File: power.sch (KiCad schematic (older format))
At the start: 21 parts

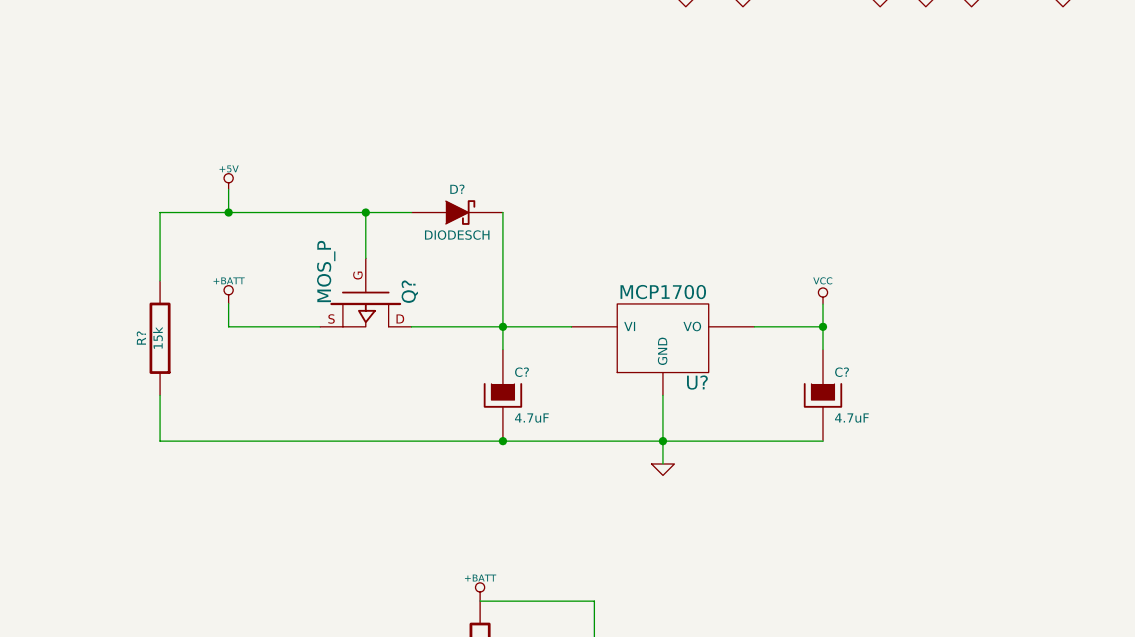
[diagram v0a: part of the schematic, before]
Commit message: Add power switch
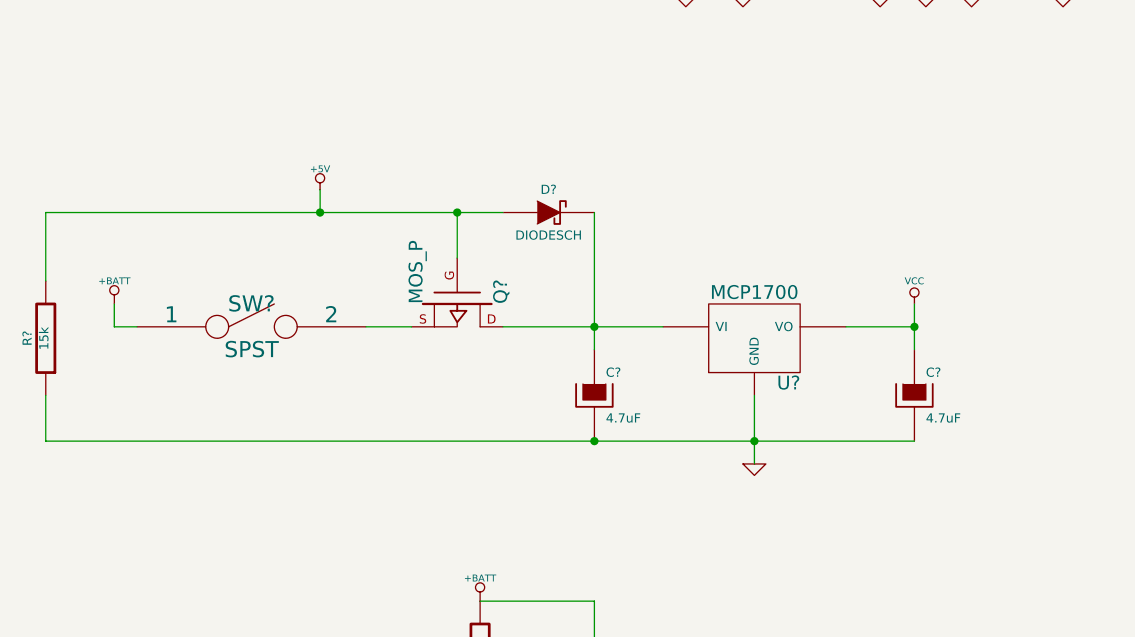
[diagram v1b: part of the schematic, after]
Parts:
- added SW?: SPST, symbol SPST
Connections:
- net +BATT: now also SW?.1; no longer Q?.S
- new net: Q?.S, SW?.2
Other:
- moved on the sheet: C?, D?, Q?, R?, U?
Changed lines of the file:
@@
 L MOS_P Q?
 U 1 1 54E64290
-P 2200 3900
-F 0 "Q?" H 2200 4090 60  0000 R CNN
-F 1 "MOS_P" H 2200 3720 60  0000 R CNN
-F 2 "" H 2200 3900 60  0000 C CNN
-F 3 "" H 2200 3900 60  0000 C CNN
-	1    2200 3900
+P 2600 3900
+F 0 "Q?" H 2600 4090 60  0000 R CNN
+F 1 "MOS_P" H 2600 3720 60  0000 R CNN
+F 2 "" H 2600 3900 60  0000 C CNN
+F 3 "" H 2600 3900 60  0000 C CNN
+	1    2600 3900
 	0    1    1    0
 $EndComp
@@
 L +BATT #PWR?
 U 1 1 54E64297
-P 1600 3900
-F 0 "#PWR?" H 1600 3850 20  0001 C CNN
-F 1 "+BATT" H 1600 4000 30  0000 C CNN
-F 2 "" H 1600 3900 60  0000 C CNN
-F 3 "" H 1600 3900 60  0000 C CNN
-	1    1600 3900
+P 1100 3900
+F 0 "#PWR?" H 1100 3850 20  0001 C CNN
+F 1 "+BATT" H 1100 4000 30  0000 C CNN
+F 2 "" H 1100 3900 60  0000 C CNN
+F 3 "" H 1100 3900 60  0000 C CNN
+	1    1100 3900
 	1    0    0    -1
 $EndComp
@@
 L CP C?
 U 1 1 54E6429D
-P 2800 4300
-F 0 "C?" H 2850 4400 40  0000 L CNN
-F 1 "4.7uF" H 2850 4200 40  0000 L CNN
-F 2 "" H 2900 4150 30  0000 C CNN
-F 3 "" H 2800 4300 300 0000 C CNN
-	1    2800 4300
+P 3200 4300
+F 0 "C?" H 3250 4400 40  0000 L CNN
+F 1 "4.7uF" H 3250 4200 40  0000 L CNN
+F 2 "" H 3300 4150 30  0000 C CNN
+F 3 "" H 3200 4300 300 0000 C CNN
+	1    3200 4300
 	1    0    0    -1
 $EndComp
@@
 L DIODESCH D?
 U 1 1 54E642A4
-P 2600 3500
-F 0 "D?" H 2600 3600 40  0000 C CNN
-F 1 "DIODESCH" H 2600 3400 40  0000 C CNN
-F 2 "" H 2600 3500 60  0000 C CNN
-F 3 "" H 2600 3500 60  0000 C CNN
-	1    2600 3500
+P 3000 3500
+F 0 "D?" H 3000 3600 40  0000 C CNN
+F 1 "DIODESCH" H 3000 3400 40  0000 C CNN
+F 2 "" H 3000 3500 60  0000 C CNN
+F 3 "" H 3000 3500 60  0000 C CNN
+	1    3000 3500
 	1    0    0    -1
 $EndComp
@@
 L MCP1700 U?
 U 1 1 54E642AB
-P 3500 4050
-F 0 "U?" H 3650 3854 60  0000 C CNN
-F 1 "MCP1700" H 3500 4250 60  0000 C CNN
-F 2 "" H 3500 4050 60  0000 C CNN
-F 3 "" H 3500 4050 60  0000 C CNN
-	1    3500 4050
+P 3900 4050
+F 0 "U?" H 4050 3854 60  0000 C CNN
+F 1 "MCP1700" H 3900 4250 60  0000 C CNN
+F 2 "" H 3900 4050 60  0000 C CNN
+F 3 "" H 3900 4050 60  0000 C CNN
+	1    3900 4050
 	1    0    0    -1
 $EndComp
@@
 L VCC #PWR?
 U 1 1 54E642B2
-P 4200 3900
-F 0 "#PWR?" H 4200 4000 30  0001 C CNN
-F 1 "VCC" H 4200 4000 30  0000 C CNN
-F 2 "" H 4200 3900 60  0000 C CNN
-F 3 "" H 4200 3900 60  0000 C CNN
-	1    4200 3900
+P 4600 3900
+F 0 "#PWR?" H 4600 4000 30  0001 C CNN
+F 1 "VCC" H 4600 4000 30  0000 C CNN
+F 2 "" H 4600 3900 60  0000 C CNN
+F 3 "" H 4600 3900 60  0000 C CNN
+	1    4600 3900
 	1    0    0    -1
 $EndComp
 Wire Wire Line
-	2400 4000 3100 4000
+	2800 4000 3500 4000
 Wire Wire Line
-	2800 3500 2800 4100
-Connection ~ 2800 4000
+	3200 3500 3200 4100
+Connection ~ 3200 4000
 Wire Wire Line
-	1600 3900 1600 4000
+	1100 3900 1100 4000
 Wire Wire Line
-	1600 4000 2000 4000
+	2600 3700 2600 3500
 Wire Wire Line
-	2200 3700 2200 3500
-Wire Wire Line
-	1300 3500 2400 3500
+	800  3500 2800 3500
 $Comp
 L +5V #PWR?
 U 1 1 54E642BF
-P 1600 3400
-F 0 "#PWR?" H 1600 3490 20  0001 C CNN
-F 1 "+5V" H 1600 3490 30  0000 C CNN
-F 2 "" H 1600 3400 60  0000 C CNN
-F 3 "" H 1600 3400 60  0000 C CNN
-	1    1600 3400
+P 2000 3400
+F 0 "#PWR?" H 2000 3490 20  0001 C CNN
+F 1 "+5V" H 2000 3490 30  0000 C CNN
+F 2 "" H 2000 3400 60  0000 C CNN
+F 3 "" H 2000 3400 60  0000 C CNN
+	1    2000 3400
 	1    0    0    -1
 $EndComp
 Wire Wire Line
-	1600 3400 1600 3500
-Connection ~ 2200 3500
+	2000 3400 2000 3500
+Connection ~ 2600 3500
 Wire Wire Line
-	3900 4000 4200 4000
+	4300 4000 4600 4000
 Wire Wire Line
-	4200 3900 4200 4100
+	4600 3900 4600 4100
 $Comp
 L GND #PWR?
 U 1 1 54E642C9
-P 3500 4600
-F 0 "#PWR?" H 3500 4600 30  0001 C CNN
-F 1 "GND" H 3500 4530 30  0001 C CNN
-F 2 "" H 3500 4600 60  0000 C CNN
-F 3 "" H 3500 4600 60  0000 C CNN
-	1    3500 4600
+P 3900 4600
+F 0 "#PWR?" H 3900 4600 30  0001 C CNN
+F 1 "GND" H 3900 4530 30  0001 C CNN
+F 2 "" H 3900 4600 60  0000 C CNN
+F 3 "" H 3900 4600 60  0000 C CNN
+	1    3900 4600
 	1    0    0    -1
 $EndComp
 Wire Wire Line
-	1300 4500 4200 4500
+	800  4500 4600 4500
 Wire Wire Line
-	3500 4300 3500 4600
-Connection ~ 3500 4500
+	3900 4300 3900 4600
+Connection ~ 3900 4500
 $Comp
 L R R?
 U 1 1 54E642D2
-P 1300 4050
-F 0 "R?" V 1380 4050 40  0000 C CNN
-F 1 "15k" V 1307 4051 40  0000 C CNN
-F 2 "" V 1230 4050 30  0000 C CNN
-F 3 "" H 1300 4050 30  0000 C CNN
-	1    1300 4050
+P 800 4050
+F 0 "R?" V 880 4050 40  0000 C CNN
+F 1 "15k" V 807 4051 40  0000 C CNN
+F 2 "" V 730 4050 30  0000 C CNN
+F 3 "" H 800 4050 30  0000 C CNN
+	1    800  4050
 	-1   0    0    1
 $EndComp
 Wire Wire Line
-	1300 3800 1300 3500
-Connection ~ 1600 3500
+	800  3800 800  3500
+Connection ~ 2000 3500
 Wire Wire Line
-	1300 4300 1300 4500
-Connection ~ 2800 4500
+	800  4300 800  4500
+Connection ~ 3200 4500
 $Comp
 L CP C?
 U 1 1 54E642DD
-P 4200 4300
-F 0 "C?" H 4250 4400 40  0000 L CNN
-F 1 "4.7uF" H 4250 4200 40  0000 L CNN
-F 2 "" H 4300 4150 30  0000 C CNN
-F 3 "" H 4200 4300 300 0000 C CNN
-	1    4200 4300
+P 4600 4300
+F 0 "C?" H 4650 4400 40  0000 L CNN
+F 1 "4.7uF" H 4650 4200 40  0000 L CNN
+F 2 "" H 4700 4150 30  0000 C CNN
+F 3 "" H 4600 4300 300 0000 C CNN
+	1    4600 4300
 	1    0    0    -1
 $EndComp
-Connection ~ 4200 4000
+Connection ~ 4600 4000
+$Comp
+L SPST SW?
+U 1 1 54E81B6B
+P 1700 4000
+F 0 "SW?" H 1700 4100 70  0000 C CNN
+F 1 "SPST" H 1700 3900 70  0000 C CNN
+F 2 "" H 1700 4000 60  0000 C CNN
+F 3 "" H 1700 4000 60  0000 C CNN
+	1    1700 4000
+	1    0    0    -1
+$EndComp
+Wire Wire Line
+	1100 4000 1200 4000
+Wire Wire Line
+	2200 4000 2400 4000
 $EndSCHEMATC
